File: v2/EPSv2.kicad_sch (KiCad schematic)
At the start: 38 parts, among them J1 Conn_01x03, J2 Conn_01x03, J3 Conn_01x02, J4 5037630491, J5 2P 21700 Cell Holder, J6 5037630491, J7 1053091102, J8 1053091102, J9 1053091102

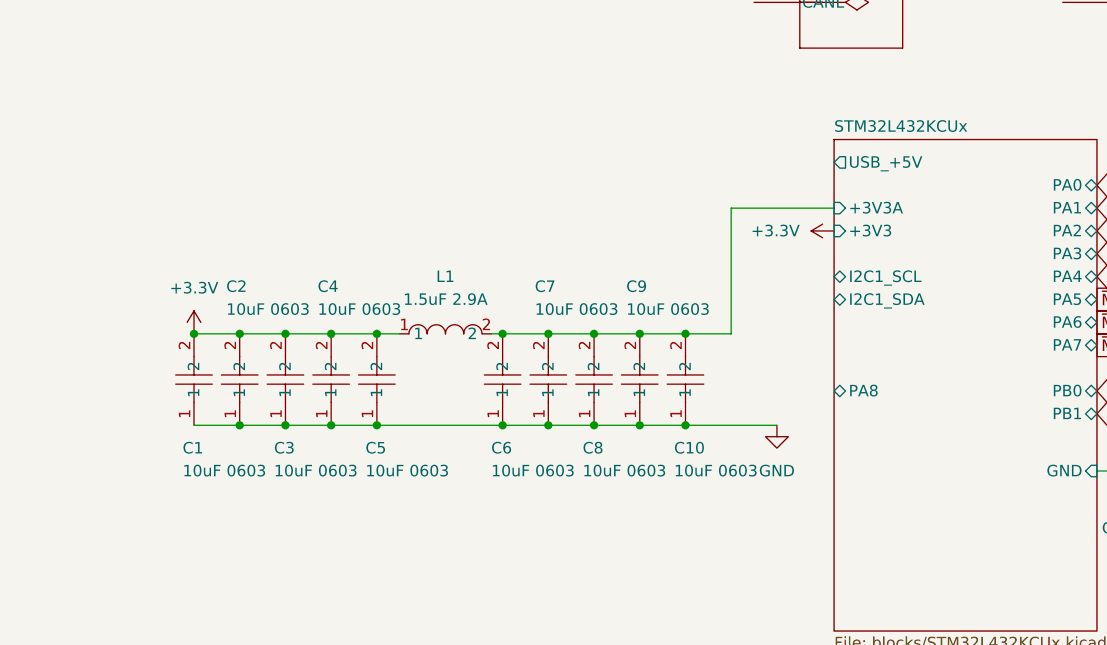
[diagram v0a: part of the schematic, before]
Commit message: battery charging routing
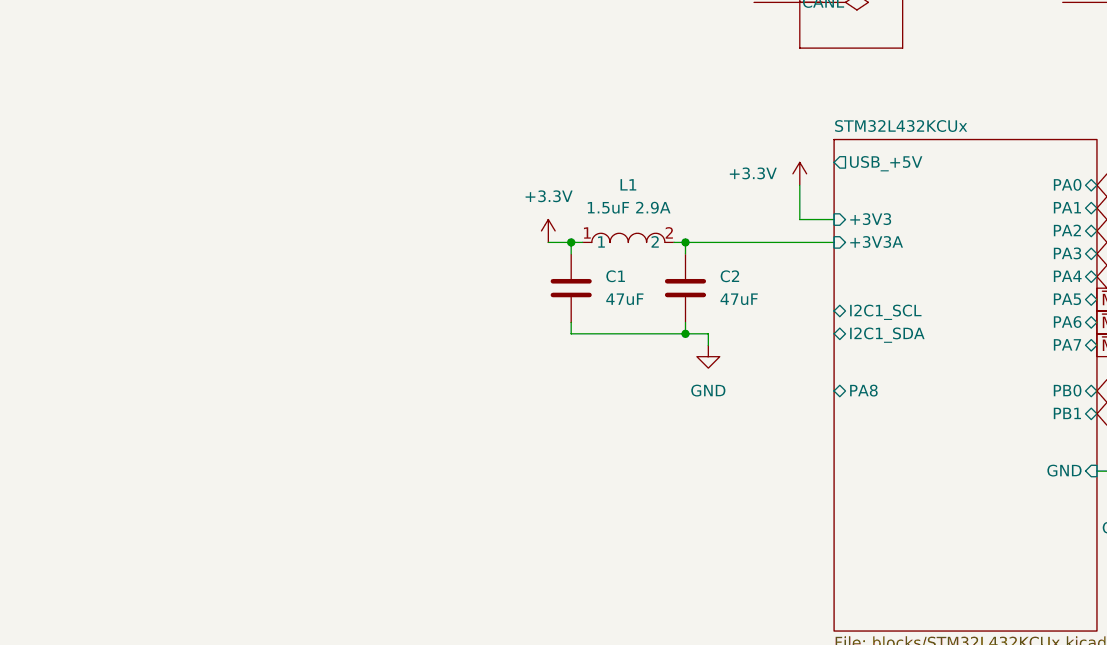
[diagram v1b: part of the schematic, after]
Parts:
- removed C1, C10, C2, C3, C4, C5, C6, C7, C8, C9: 10uF 0603, Rocketry_Easyeda:C0603, symbol Rocketry_Easyeda:CL10A106KP8NNNC (10uF 0603)
- added C1, C2: 47uF, Capacitor_SMD:C_0603_1608Metric, symbol Device:C
- J4, J6: footprint CON_5037630491 -> Rocketry_Manual:CON_5037630491
- J7, J8, J9: footprint CON_1053091102 -> Rocketry_Manual:CON_1053091102
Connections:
- net +3.3V: now also C1.1
- net GND: now also C1.2, C2.2
- net STM32L432KCUx/+3V3A: now also C2.1
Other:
- moved on the sheet: L1
